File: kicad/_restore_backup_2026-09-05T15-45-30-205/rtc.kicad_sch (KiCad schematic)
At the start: 4 parts, among them U7 BME280

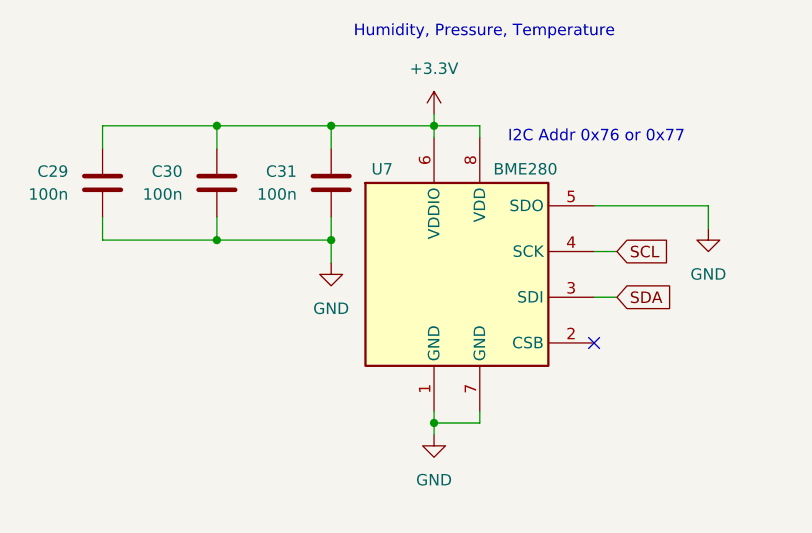
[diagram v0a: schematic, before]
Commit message: merge
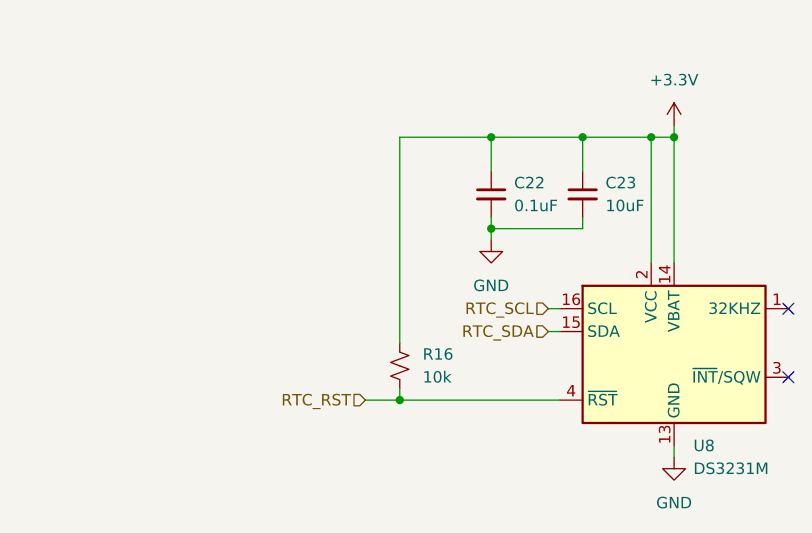
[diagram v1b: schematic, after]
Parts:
- removed C29, C30, C31: 100n, Capacitor_SMD:C_0603_1608Metric, symbol Device:C
- removed U7: BME280, Package_LGA:Bosch_LGA-8_2.5x2.5mm_P0.65mm_ClockwisePinNumbering, symbol Sensor:BME280
- added C22: 0.1uF, Capacitor_SMD:C_0805_2012Metric, symbol Device:C_Small
- added C23: 10uF, Capacitor_SMD:C_0805_2012Metric, symbol Device:C_Small
- added R16: 10k, Resistor_SMD:R_0805_2012Metric, symbol Device:R_Small_US
- added U8: DS3231M, Package_SO:SOIC-16W_7.5x10.3mm_P1.27mm, symbol Timer_RTC:DS3231M
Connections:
- net +3.3V: now also C22.1, C23.1, R16.1, U8.14 (VBAT), U8.2 (VCC)
- net GND: now also C22.2, C23.2, U8.10 (GND), U8.11 (GND), U8.12 (GND), U8.13 (GND), U8.5 (GND), U8.6 (GND), U8.7 (GND), U8.8 (GND), U8.9 (GND)
- new net RTC_RST: R16.2, U8.4 (~{RST})
- new net RTC_SCL: U8.16 (SCL)
- new net RTC_SDA: U8.15 (SDA)
- no-connect marks 1 -> 2
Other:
- note removed: "Humidity, Pressure, Temperature"
- note removed: "I2C Addr 0x76 or 0x77"
